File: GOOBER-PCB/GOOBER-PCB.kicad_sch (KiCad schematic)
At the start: 88 parts, among them J1 XT30U_F, J2 Conn_01x22, J3 Conn_01x22, J4 Conn_01x22, J5 Conn_01x22, J6 XT30U_F, J8 USB C vertical, Q3 PJD15P06A_L2_00001, Q4 AO3419, U1 TPS565208

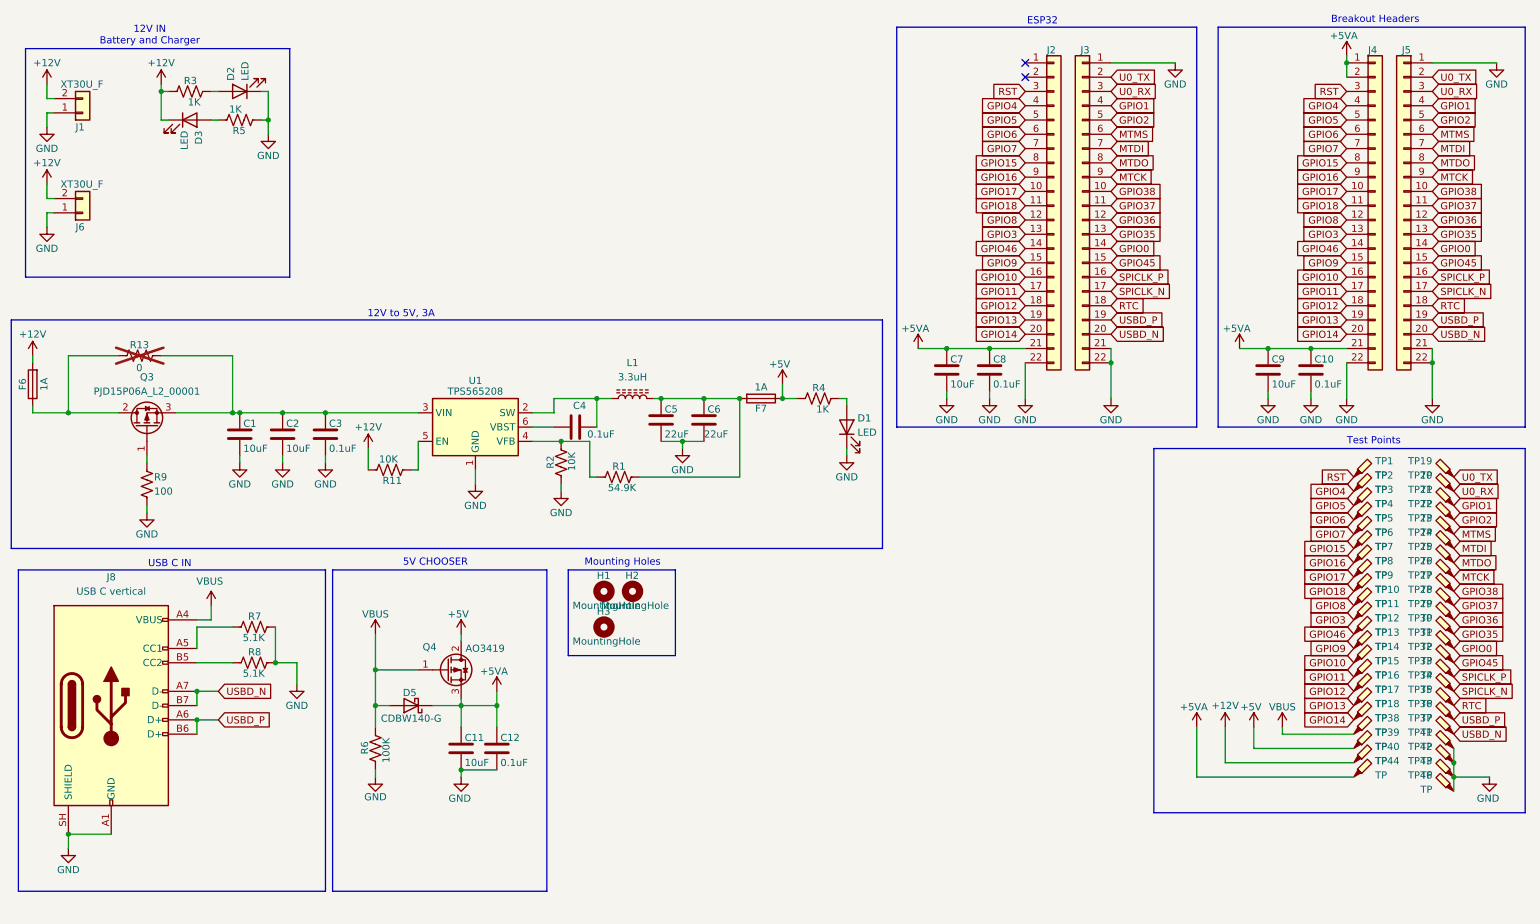
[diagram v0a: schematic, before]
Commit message: some work on pcb
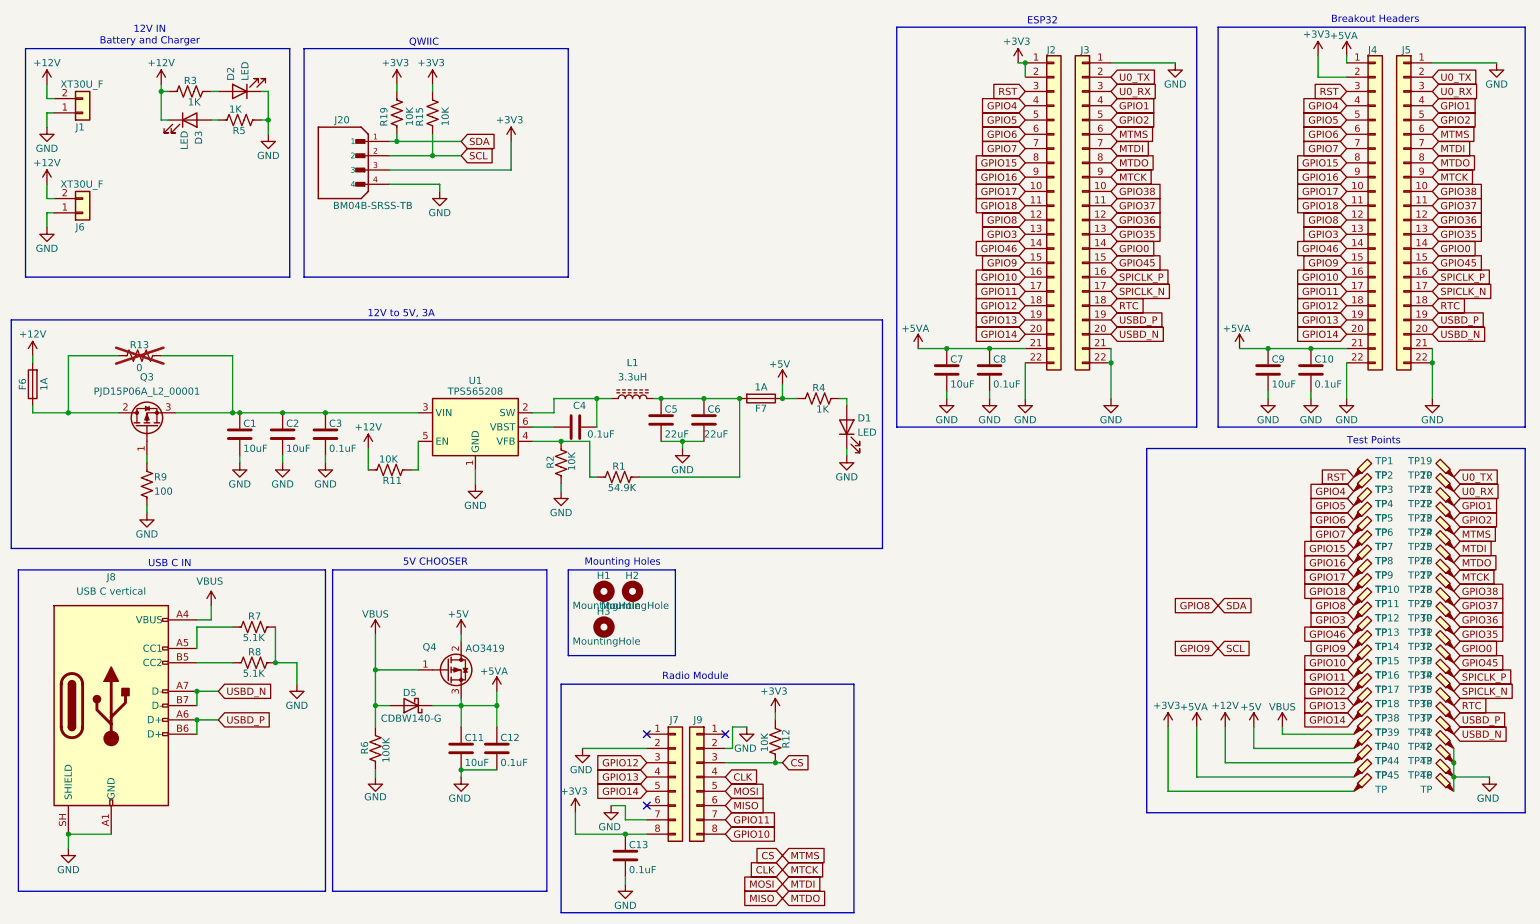
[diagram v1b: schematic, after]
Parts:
- added C13: 0.1uF, Capacitor_SMD:C_0805_2012Metric_Pad1.18x1.45mm_HandSolder, symbol Device:C
- added J20: BM04B-SRSS-TB, Connector_JST:JST_SH_BM04B-SRSS-TB_1x04-1MP_P1.00mm_Vertical, symbol QWIIC:PRT-14417
- added J7, J9: Conn_01x08, Connector_PinHeader_2.54mm:PinHeader_1x08_P2.54mm_Vertical, symbol Connector_Generic:Conn_01x08
- added R12, R15, R19: 10K, Resistor_SMD:R_0805_2012Metric_Pad1.20x1.40mm_HandSolder, symbol Device:R_US
- added TP45: TP, TestPoint:TestPoint_Keystone_5000-5004_Miniature, symbol Connector:TestPoint_Probe
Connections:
- net +5VA: no longer J4.2 (Pin_2)
- net GND: now also C13.2, J20.4, J7.2 (Pin_2), J7.7 (Pin_7), J9.2 (Pin_2)
- net GPIO10: now also J9.8 (Pin_8)
- net GPIO11: now also J9.7 (Pin_7)
- net GPIO12: now also J7.3 (Pin_3)
- net GPIO13: now also J7.4 (Pin_4)
- net GPIO14: now also J7.5 (Pin_5)
- net GPIO8: now also J20.1, R19.1
- net GPIO9: now also J20.2, R15.1
- net +3V3: now reaches J2.1 (Pin_1)
- net +3V3: now also J2.2 (Pin_2), J4.2 (Pin_2), C13.1, J20.3, J7.8 (Pin_8), R12.1, R15.2, R19.2, TP45.1
- net MTCK renamed CLK
- net CLK: now also J9.4 (Pin_4)
- net MTDI renamed MOSI
- net MOSI: now also J9.5 (Pin_5)
- net MTDO renamed MISO
- net MISO: now also J9.6 (Pin_6)
- net MTMS renamed CS
- net CS: now also J9.3 (Pin_3), R12.2
- no-connect marks 2 -> 3
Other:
- note added: "QWIIC"
- note added: "Radio Module"

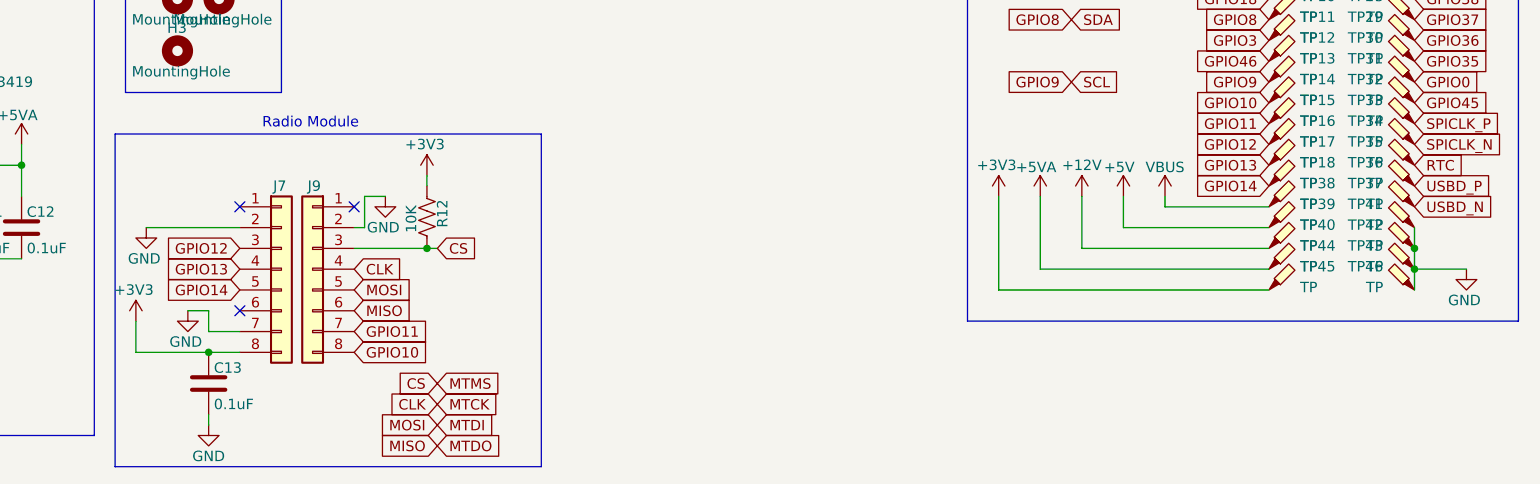
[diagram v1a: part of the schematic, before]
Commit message: first revision of goober pcb
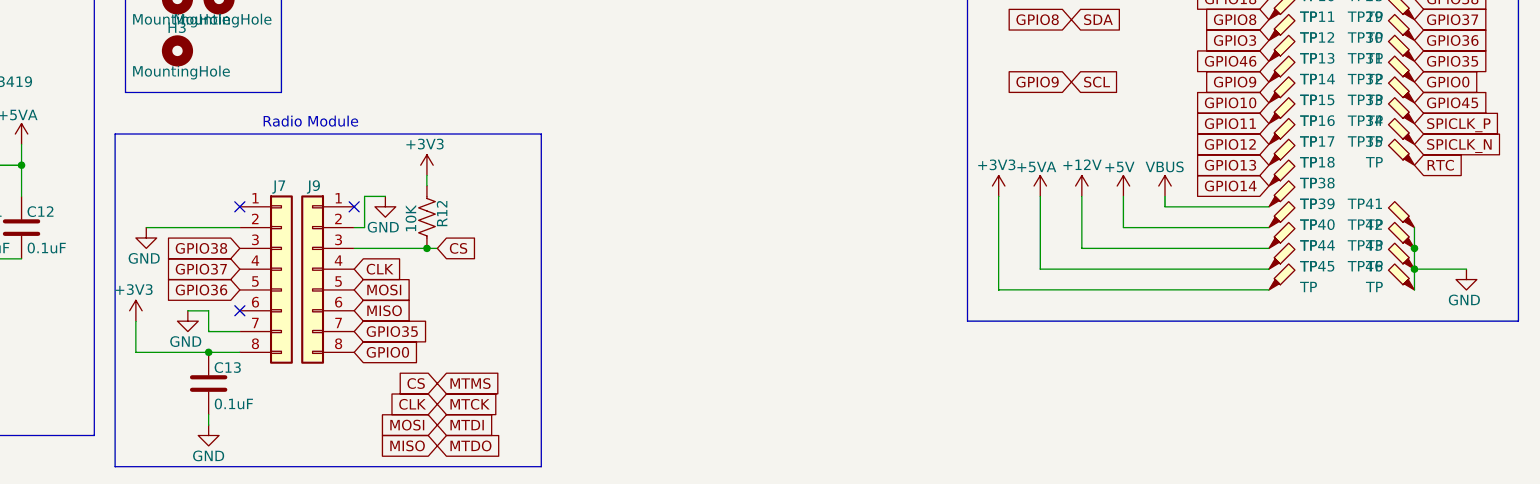
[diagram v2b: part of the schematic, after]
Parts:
- removed TP36, TP37: TP, TestPoint:TestPoint_Keystone_5000-5004_Miniature, symbol Connector:TestPoint_Probe
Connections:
- net GPIO0: now also J9.8 (Pin_8)
- net GPIO10: no longer J9.8 (Pin_8)
- net GPIO11: no longer J9.7 (Pin_7)
- net GPIO12: no longer J7.3 (Pin_3)
- net GPIO13: no longer J7.4 (Pin_4)
- net GPIO14: no longer J7.5 (Pin_5)
- net GPIO35: now also J9.7 (Pin_7)
- net GPIO36: now also J7.5 (Pin_5)
- net GPIO37: now also J7.4 (Pin_4)
- net GPIO38: now also J7.3 (Pin_3)
